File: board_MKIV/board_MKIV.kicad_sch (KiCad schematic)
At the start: 43 parts, among them J1 1757242, J2 jst-power, J3 JST -SM, J5 1770979, J6 20_pin_90, J7 20-pin-straight, U1 ESP32-DEVKITC-32D, U2 LTV-846S, U3 TLV272CDR, U4 BAT46W, U5 BA&, U6 SH-7070TB

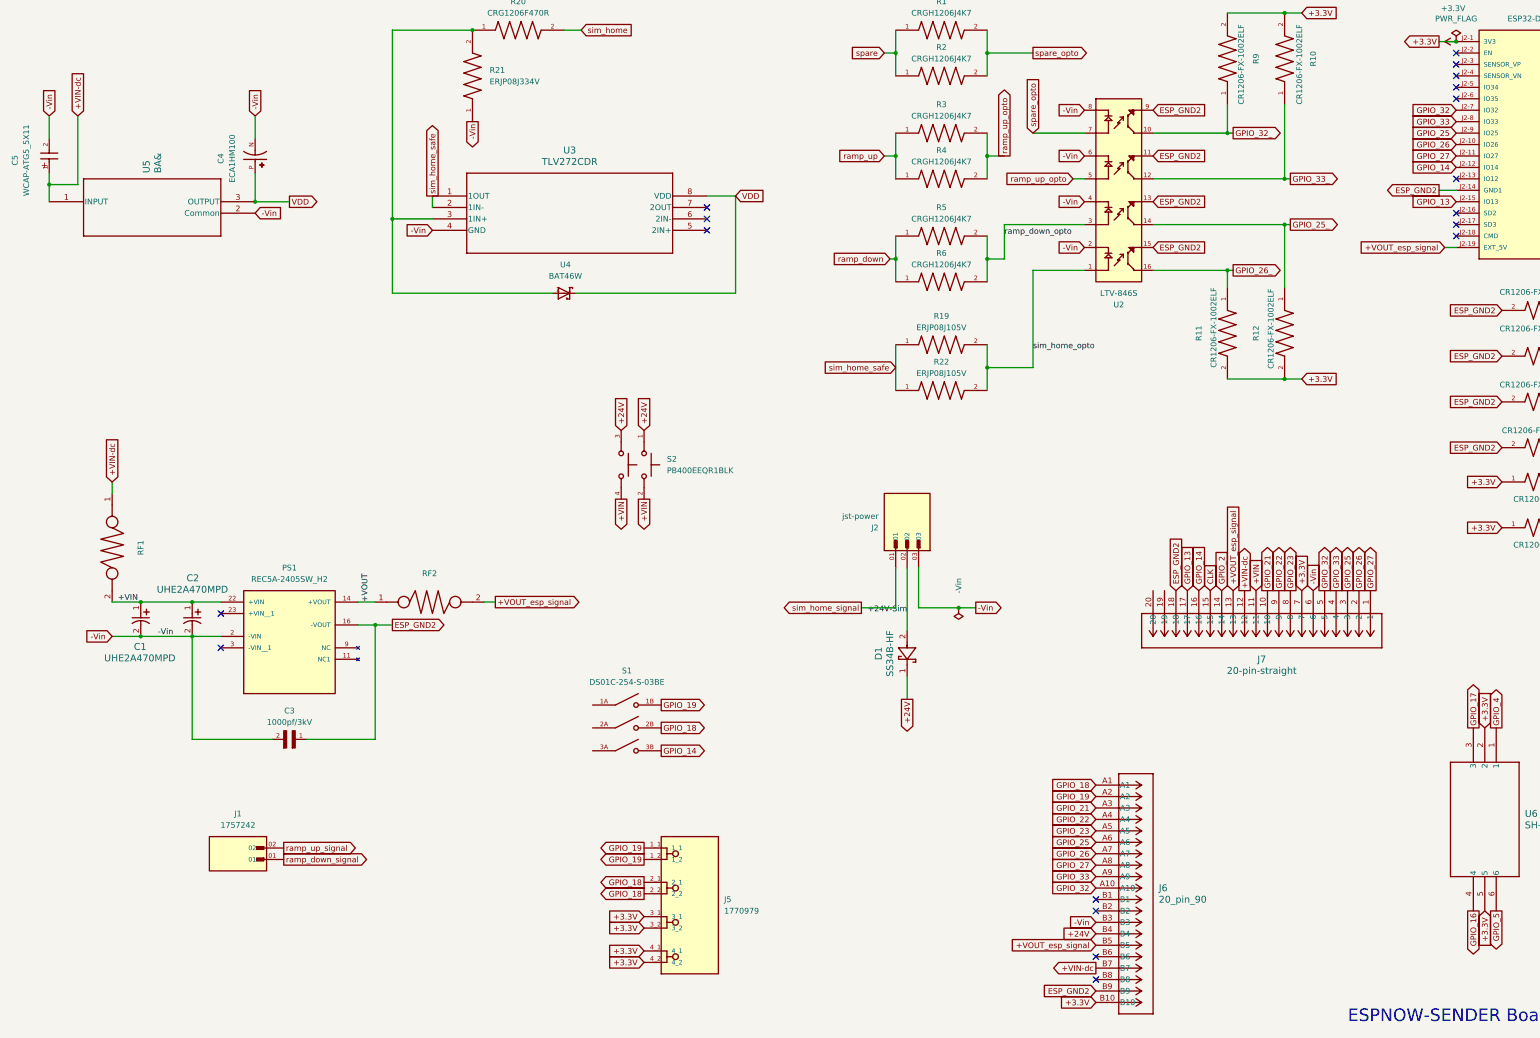
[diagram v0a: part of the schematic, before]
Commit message: update
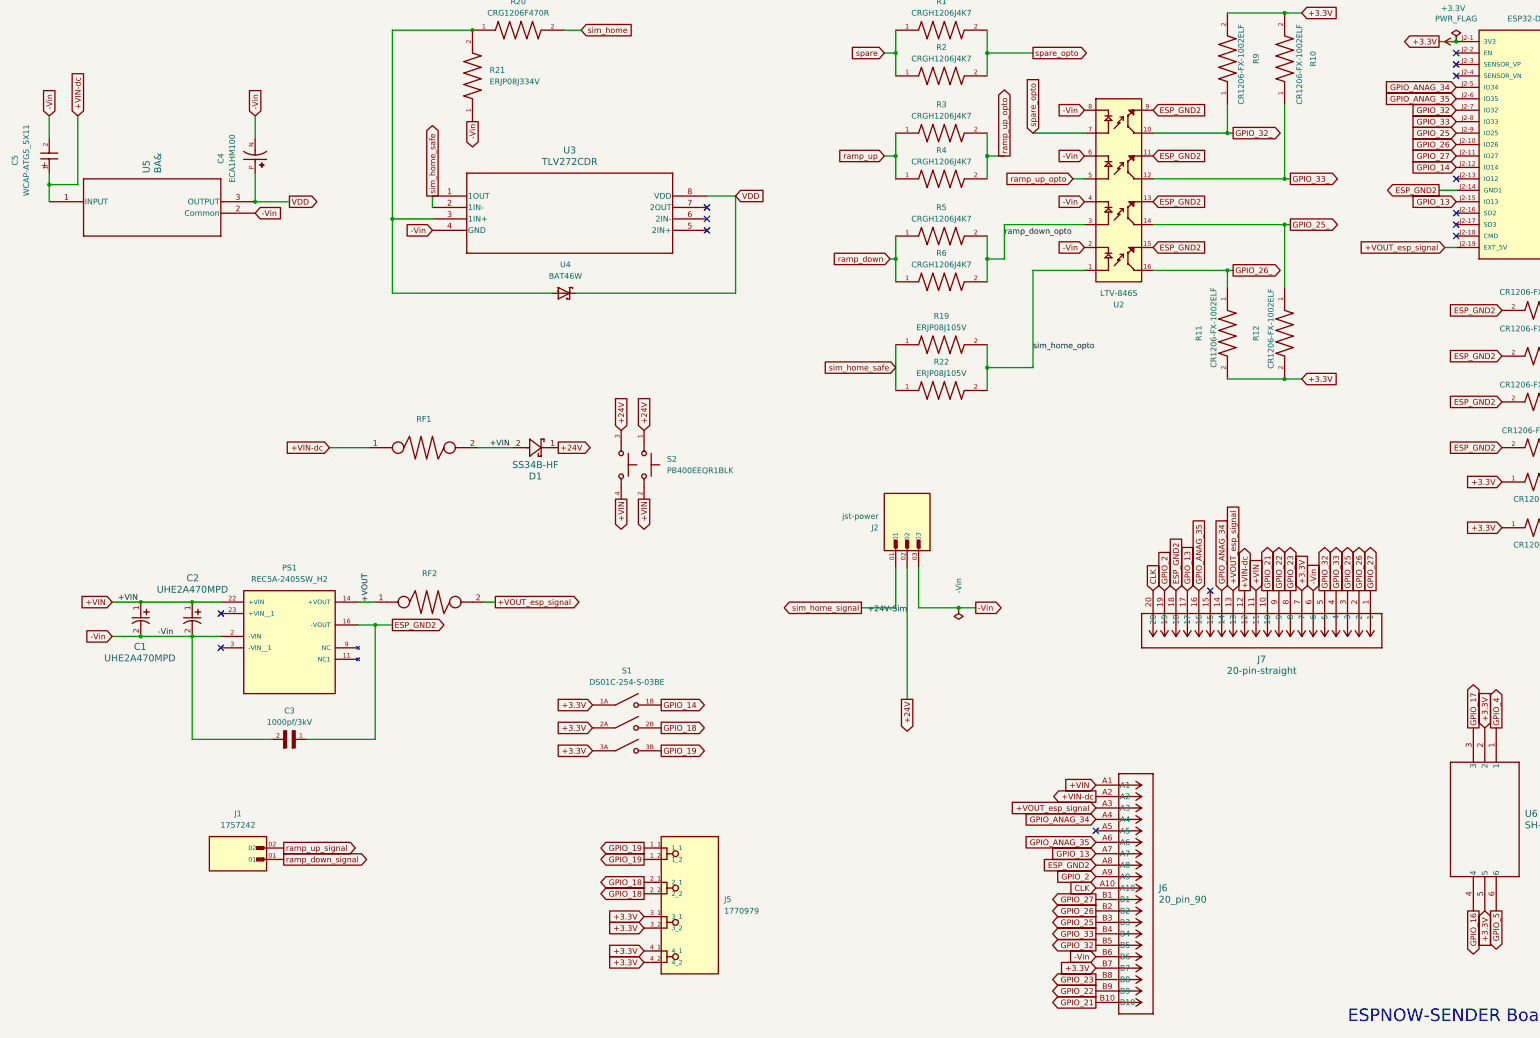
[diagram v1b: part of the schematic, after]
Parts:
- S1: footprint DS01C-254-S-03BE:SW_DS01C-254-S-03BE -> footprints:SW_DS01C-254-S-03BE
- U6: footprint SH-7070TB_7P1X7P3_NDC -> footprints:SH-7070TB_7P1X7P3_NDC
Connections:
- net +24V: now also J2.02; no longer J6.B4
- net +3.3V: now also J6.B7, S1.1A, S1.2A, S1.3A; no longer J6.B10
- net +VIN: now also D1.2, J6.A1
- net +VIN-dc: now also J6.A2; no longer J6.B7
- net +VOUT_esp_signal: now also J6.A3; no longer J6.B5
- net -Vin: now also J6.B6; no longer J6.B3
- net CLK: now also J6.A10, J7.20; no longer J7.15
- net ESP_GND2: now also J6.A8; no longer J6.B9
- net GPIO_13: now also J6.A7
- net GPIO_14: now also S1.1B; no longer J7.16, S1.3B
- net GPIO_18: no longer J6.A1
- net GPIO_19: now also S1.3B; no longer J6.A2, S1.1B
- net GPIO_2: now also J6.A9, J7.19; no longer J7.14
- net GPIO_21: now also J6.B10; no longer J6.A3
- net GPIO_22: now also J6.B9; no longer J6.A4
- net GPIO_23: now also J6.B8; no longer J6.A5
- net GPIO_25: now also J6.B3; no longer J6.A6
- net GPIO_26: now also J6.B2; no longer J6.A7
- net GPIO_27: now also J6.B1; no longer J6.A8
- net GPIO_32: now also J6.B5; no longer J6.A10
- net GPIO_33: now also J6.B4; no longer J6.A9
- net GPIO_ANAG_34: now reaches U1.J2-5 (IO34)
- net GPIO_ANAG_34: now also J6.A4, J7.14
- net GPIO_ANAG_35: now reaches U1.J2-6 (IO35)
- net GPIO_ANAG_35: now also J6.A6, J7.16
- removed net +24V-Sim: D1.2, J2.02
- no-connect marks 24 -> 20
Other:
- moved on the sheet: D1, RF1
